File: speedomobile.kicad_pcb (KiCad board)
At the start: 2 copper layers, 100 x 100 mm, 126 parts, among them J1 Conn_01x04, J10 Conn_02x02_Odd_Even, J11 Conn_02x02_Odd_Even, J12 Conn_02x02_Odd_Even, J13 Conn_02x02_Odd_Even, J14 Conn_02x02_Odd_Even, J15 Conn_02x02_Odd_Even, J16 Conn_02x02_Odd_Even, J17 Conn_02x02_Odd_Even, J18 Conn_01x02, J19 Conn_01x02, J2 Conn_01x04, J20 Conn_01x02, J21 Conn_01x02, J22 Conn_01x07, J23 Conn_01x04, J24 Conn_01x03, J25 Conn_01x03, J26 Conn_01x03, J27 Conn_01x02, J28 Conn_01x06, J29 Conn_01x02, J3 Conn_01x04, J30 Conn_01x06, J31 Conn_02x06_Odd_Even, J32 Conn_01x02, J33 Conn_01x03, J34 Conn_01x02, J35 SDCARD_breakout, J36 Conn_02x02_Odd_Even, J37 Conn_01x02, J38 Conn_01x04, J39 Conn_02x02_Odd_Even, J4 Conn_01x04, J5 Conn_01x05, J6 Conn_01x04, J7 Conn_01x07, J8 Conn_01x03, J9 Conn_Coaxial, Q1 DMT6012LSS, Q2 DMT6012LSS, SW1 SW_Push, U1 MCP1501-33xCH, U10 NEO-M9N, U11 PCF8574, U12 PCF8574, U13 TCA9617A, U2 SC0918, U3 74AHCT367, U4 BTS4140N, U5 CD74HC4067M, U6 MCS1802, U7 MCS1802, U8 V48SD, U9 adafruit_LSM9DS1

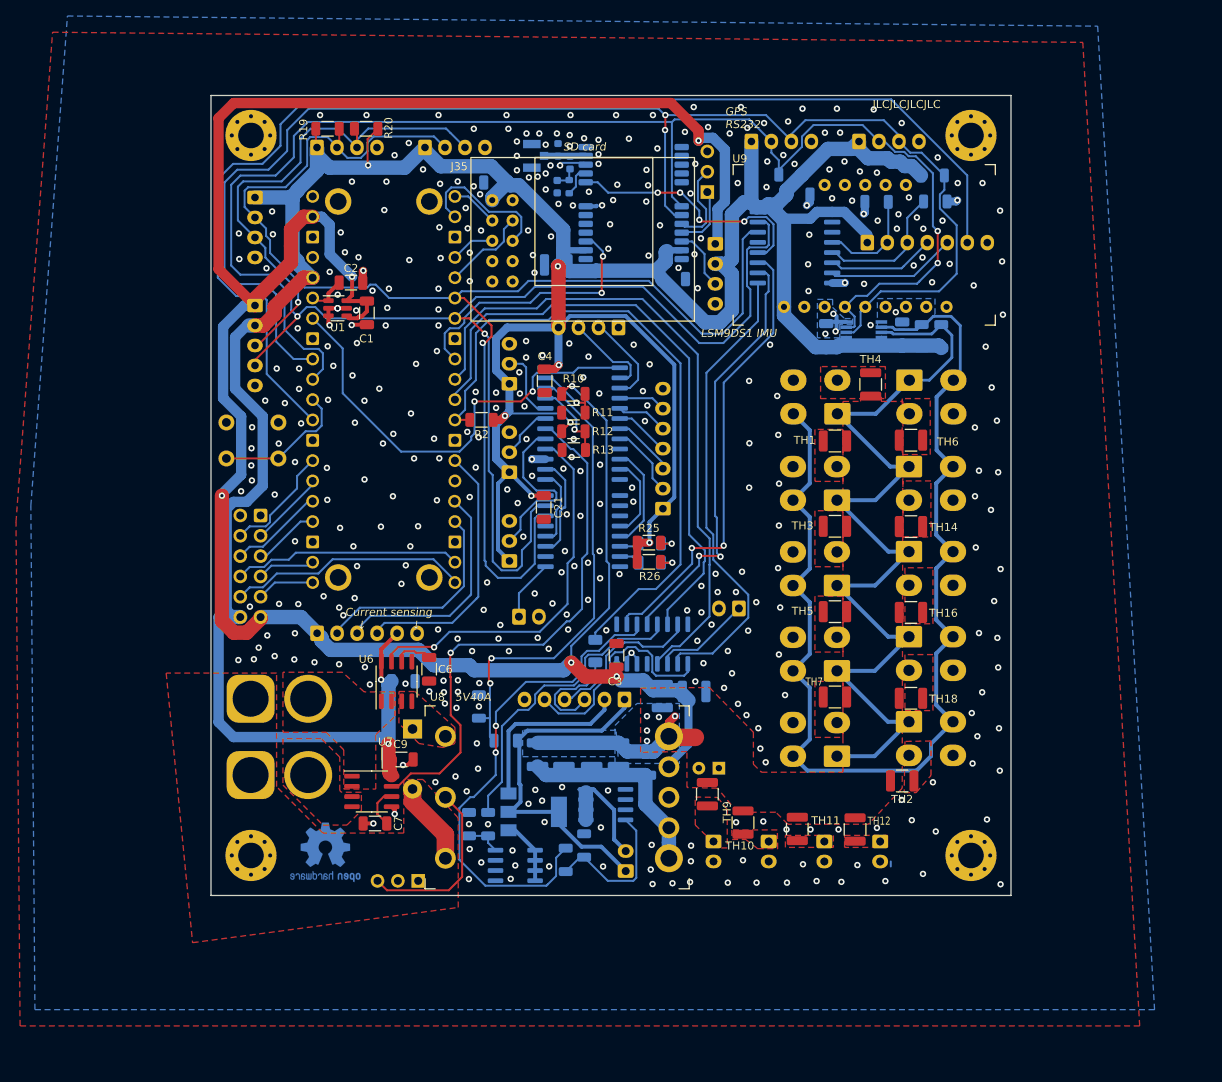
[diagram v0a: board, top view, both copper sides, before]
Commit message: Prepare for merging
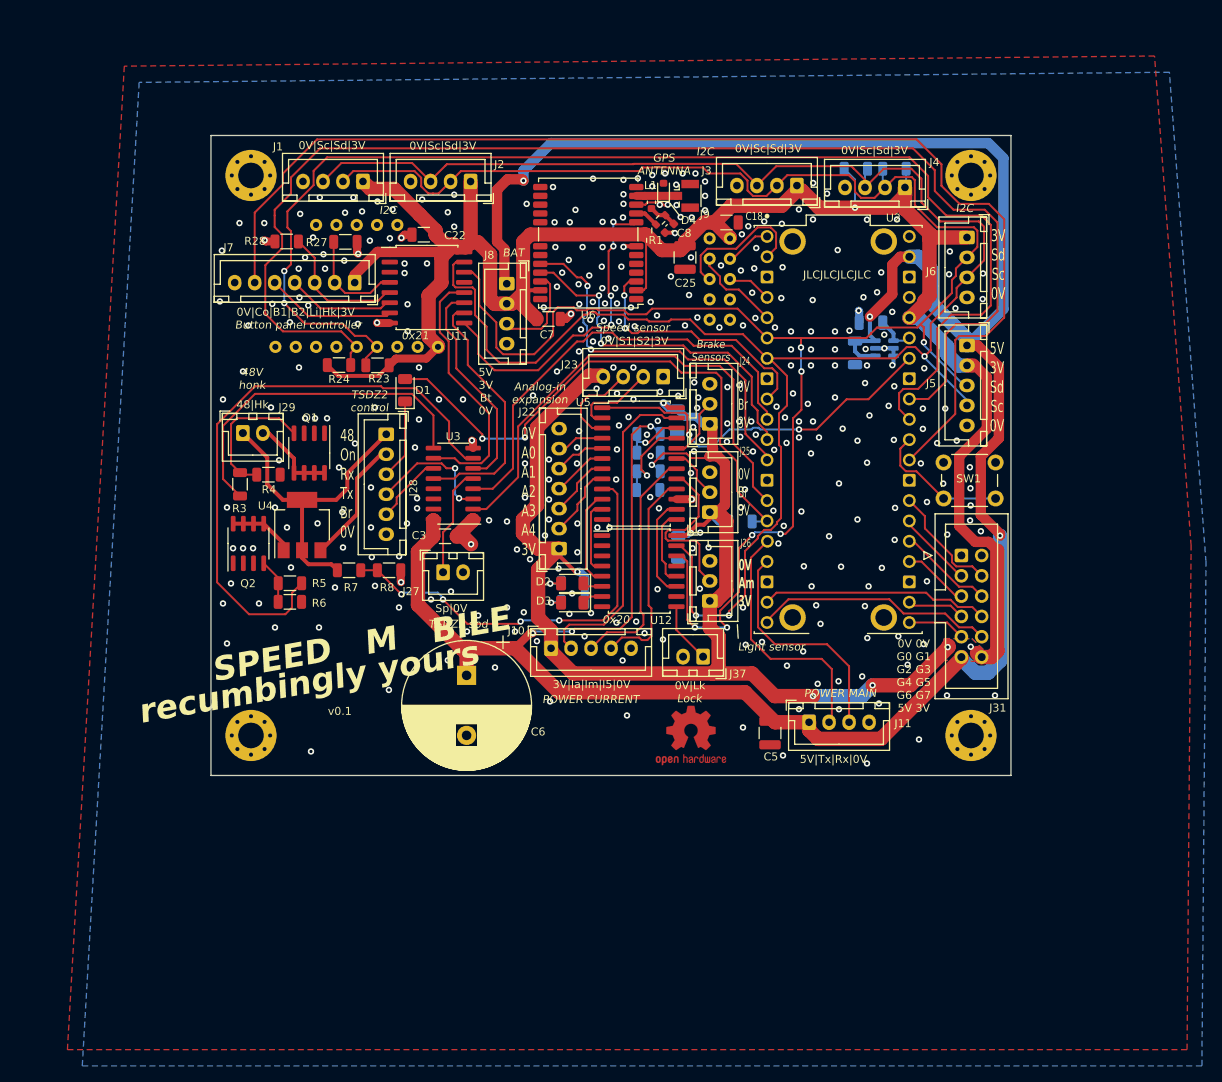
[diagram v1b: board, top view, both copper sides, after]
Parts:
- removed C10, C11, C12, C13, C15, C16: 22u, Capacitor_SMD:C_1210_3225Metric
- removed C14: 100u, Capacitor_THT:CP_Radial_D6.3mm_P2.50mm
- removed C19, C9: 1u, Capacitor_SMD:C_1206_3216Metric
- removed C20: 100n, Capacitor_SMD:C_0603_1608Metric
- removed C23, C24: 100n, Capacitor_SMD:C_1206_3216Metric
- removed J12, J13, J14, J15, J16, J17, J36, J39: Conn_02x02_Odd_Even, Connector_Molex:Molex_Mini-Fit_Jr_5566-04A_2x02_P4.20mm_Vertical
- removed J18, J19, J20, J21: Conn_01x02, Connector_JST:JST_XH_B2B-XH-A_1x02_P2.50mm_Vertical
- removed J30: Conn_01x06, Connector_JST:JST_XH_B6B-XH-A_1x06_P2.50mm_Vertical
- removed J32: Conn_01x02, Connector_AMASS:AMASS_XT60-M_1x02_P7.20mm_Vertical
- removed J33: Conn_01x03, Connector_PinHeader_2.54mm:PinHeader_1x03_P2.54mm_Vertical
- removed J34: Conn_01x02, Connector_AMASS:AMASS_XT60-F_1x02_P7.20mm_Vertical
- removed J38: Conn_01x04, Connector_JST:JST_XH_B4B-XH-A_1x04_P2.50mm_Vertical
- removed R18: 20, Resistor_SMD:R_0603_1608Metric
- removed R29: 330, Resistor_SMD:R_1206_3216Metric
- removed TH1, TH14, TH16, TH18, TH2, TH3, TH4, TH5, TH6, TH7: 7,5A, Resistor_SMD:R_1210_3225Metric
- removed TH10, TH11, TH12, TH13, TH9: 3A, Resistor_SMD:R_1210_3225Metric
- removed U10: NEO-M9N, RF_GPS:ublox_NEO
- removed U13: TCA9617A, Package_SO:VSSOP-8_3.0x3.0mm_P0.65mm
- removed U7: MCS1802, Package_SO:SOIC-8_3.9x4.9mm_P1.27mm
- removed U8: V48SD, additional:V48D
- C1, C2, C21, C4, H1, H2, H3, H4, J35, R10, R11, R12, R13, R19, R2, R20, R25, R26, U1, U9: moved to B.Cu
- C18, C22, C25, D1, D2, D3, D4, J1, J2, J22, J27, J28, J29, J3, J31, J37, J4, J5, J6, J7, J9, L1, Q1, Q2, R23, R24, R27, R28, R3, R4, R5, R6, R7, R8, SW1, SYMB1, U11, U12, U2, U3, U4, U5: moved to F.Cu
- C5: value 220u -> 22u; footprint Capacitor_THT:CP_Radial_D16.0mm_P7.50mm -> Capacitor_SMD:C_1210_3225Metric; moved to F.Cu
- C6: value 1u -> 220u; footprint Capacitor_SMD:C_1206_3216Metric -> Capacitor_THT:CP_Radial_D16.0mm_P7.50mm
- C8: value 1u -> 100n; footprint Capacitor_SMD:C_1206_3216Metric -> Capacitor_SMD:C_0603_1608Metric; moved to F.Cu
- J10: value Conn_02x02_Odd_Even -> Conn_01x05; footprint Connector_Molex:Molex_Mini-Fit_Jr_5566-04A_2x02_P4.20mm_Vertical -> Connector_JST:JST_XH_B5B-XH-A_1x05_P2.50mm_Vertical; moved to F.Cu
- J11: value Conn_02x02_Odd_Even -> JST_XH; footprint Connector_Molex:Molex_Mini-Fit_Jr_5566-04A_2x02_P4.20mm_Vertical -> Connector_JST:JST_XH_B4B-XH-A_1x04_P2.50mm_Vertical; moved to F.Cu
- J23: value Conn_01x04 -> XHB4B; moved to F.Cu
- J24, J25, J26: value Conn_01x03 -> XHB3B; moved to F.Cu
- J8: value Conn_01x03 -> Conn_01x04; footprint Connector_PinHeader_2.54mm:PinHeader_1x03_P2.54mm_Vertical -> Connector_JST:JST_XH_B4B-XH-A_1x04_P2.50mm_Vertical; moved to F.Cu
- R1: value 330 -> 20; footprint Resistor_SMD:R_1206_3216Metric -> Resistor_SMD:R_0603_1608Metric; moved to F.Cu
- U6: value MCS1802 -> NEO-M9N; footprint Package_SO:SOIC-8_3.9x4.9mm_P1.27mm -> RF_GPS:ublox_NEO
- moved H1 91.2 mm to (180.0, 110.0), turned to 180 degrees
- moved H2 91.2 mm to (90.0, 110.0), turned to 180 degrees
- moved H3 90.1 mm to (90.0, 40.0), turned to 180 degrees
- moved H4 90.1 mm to (180.0, 40.0), turned to 180 degrees
- moved J5 89.1 mm to (179.5, 61.2)
- moved J6 89.1 mm to (179.5, 47.8)
- moved J31 87.7 mm to (178.8, 87.5), turned to 0 degrees
- moved SW1 83.3 mm to (176.6, 75.9), turned to 0 degrees
- moved R28 81.2 mm to (94.5, 48.2), turned to 180 degrees
- moved R24 77.9 mm to (101.0, 63.7)
- moved J4 73.7 mm to (171.8, 41.5), turned to 180 degrees
- moved J29 72.7 mm to (89.0, 72.2), turned to 0 degrees
- moved R19 71.0 mm to (170.4, 39.2), turned to 180 degrees
- moved U1 68.5 mm to (169.2, 61.6), turned to 180 degrees
- moved C7 66.7 mm to (127.2, 57.9), turned to 0 degrees
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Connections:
- net /VREF renamed +3.3VA
- net Net-(J29-Pin_2) renamed /HONK_48V
- C5 pad 1: /power/Dcdc -> +5VL
- C5 pad 2: -BATT -> GND
- C6 pad 1: Net-(U6-FILTER) -> +5VL
- C7 pad 1: Net-(U7-FILTER) -> +3V3
- C8 pad 1: +3V3 -> Net-(C8-Pad1)
- D4 pad 1: /I2C devices/RF_GPS -> /GPS/RF_GPS
- J1 pad 2: /FAST_SDA -> /SDA
- J1 pad 3: /FAST_SCL -> /SCL
- J10 pad 1: /I2C devices/led ribbon/FAST_SCL_5V -> +3V3
- J10 pad 2: /I2C devices/led ribbon/LED1 -> /Analog input/Iaux
- J10 pad 3: /I2C devices/led ribbon/FAST_SDA_5V -> /Analog input/Imotor
- J10 pad 4: GND -> /Analog input/I5V
- J11 pad 1: /I2C devices/led ribbon/FAST_SCL_5V -> +5VL
- J11 pad 2: /I2C devices/led ribbon/LED2 -> /UARTTX
- J11 pad 3: /I2C devices/led ribbon/FAST_SDA_5V -> /UARTRX
- J2 pad 2: /FAST_SDA -> /SDA
- J2 pad 3: /FAST_SCL -> /SCL
- J8 pad 1: Net-(J8-Pin_1) -> +5VL
- J8 pad 2: Net-(J8-Pin_2) -> +3V3
- J8 pad 3: GND -> Net-(J8-Pin_3)
- J9 pad 1: /I2C devices/RF_GPS -> /GPS/RF_GPS
- L1 pad 1: Net-(C20-Pad1) -> Net-(C8-Pad1)
- L1 pad 2: /I2C devices/RF_GPS -> /GPS/RF_GPS
- R1 pad 1: +3V3 -> Net-(U6-VCC_RF)
- R1 pad 2: /I2C devices/led ribbon/FAST_SCL_5V -> Net-(C8-Pad1)
- U11 pad 10: /TSDZ2_ON -> /TSDZ2_BRAKE
- U11 pad 11: /HONK -> /TSDZ2_ON
- U11 pad 12: /I2C devices/RESET_M9N -> /HONK
- U11 pad 9: /TSDZ2_BRAKE -> /RESET_M9N
- U2 pad 11: /TSDZ2_TX -> /GPS_TX
- U2 pad 12: /TSDZ2_RX -> /GPS_RX
- U2 pad 14: /AUX -> /TSDZ2_TX
- U2 pad 15: unconnected-(U2-I2C1SCL/SPI1TX/GP11-Pad15) -> /TSDZ2_RX
- U3 pad 10: /TSDZ2_BRAKE -> /HONK
- U3 pad 11: /VSPEED_5V -> /TSDZ2_BRAKE_5V
- U3 pad 12: /VSPEED -> /TSDZ2_BRAKE
- U3 pad 2: /HONK -> /TSDZ2_TX
- U3 pad 3: /HONK_5V -> /TSDZ2_TX_5V
- U3 pad 4: /TSDZ2_ON -> /VSPEED
- U3 pad 5: /TSDZ2_ON_5V -> /VSPEED_5V
- U3 pad 6: /TSDZ2_TX -> /TSDZ2_ON
- U3 pad 7: /TSDZ2_TX_5V -> /TSDZ2_ON_5V
- U3 pad 9: /TSDZ2_BRAKE_5V -> /HONK_5V
- U5 pad 16: /I5V -> /Analog input/I5V
- U5 pad 18: /Imotor -> /Analog input/Imotor
- U5 pad 2: /Analog input/ADC_SPEED1 -> /Analog input/ADC_SPEED2
- U5 pad 22: /Analog input/VBATADC -> /Analog input/U5V
- U5 pad 23: /Analog input/U5V -> /Analog input/Iaux
- U5 pad 3: /Analog input/ADC_SPEED2 -> /Analog input/ADC_SPEED1
- U5 pad 9: unconnected-(U5-I0-Pad9) -> /Analog input/VBATADC
- U6 pad 1: +BATT -> unconnected-(U6-~{SAFEBOOT}-Pad1)
- U6 pad 2: +BATT -> +3V3
- U6 pad 3: /power/Dcdc -> /PPS
- U6 pad 4: /power/Dcdc -> unconnected-(U6-EXTINT-Pad4)
- U6 pad 5: GND -> unconnected-(U6-USB_DM-Pad5)
- U6 pad 6: Net-(U6-FILTER) -> unconnected-(U6-USB_DP-Pad6)
- U6 pad 7: /I5V -> GND
- U6 pad 8: +3V3 -> /RESET_M9N
- U9 pad 6: GND -> unconnected-(U9-CS_AG-Pad6)
- U9 pad 7: GND -> unconnected-(U9-CS_M-Pad7)
- U9 pad 8: GND -> unconnected-(U9-MISO_AG-Pad8)
- U9 pad 9: GND -> unconnected-(U9-MISO_M-Pad9)
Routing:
- net /I2C devices/led ribbon/FAST_SDA_5V: track 141.9 -> 0.00 mm
- net /I2C devices/led ribbon/FAST_SCL_5V: track 119.6 -> 0.00 mm
- net /Imotor: track 67.6 -> 0.00 mm, vias 1 -> 0
- net /SDA: track 184.4 -> 251.9 mm, vias 2 -> 7
- net /SCL: track 192.9 -> 254.8 mm, vias 2 -> 3
- net /GPS_RX: track 0.00 -> 47.8 mm, vias 0 -> 2
- net /I5V: track 47.4 -> 0.00 mm, vias 1 -> 0
- net /GPS_TX: track 0.00 -> 44.7 mm, vias 0 -> 2
- net /RESET_M9N: track 0.00 -> 40.9 mm, vias 0 -> 4
- net /Analog input/Iaux: track 0.00 -> 40.7 mm
- net /TSDZ2_ON_5V: track 38.6 -> 73.9 mm
- net /AUX: track 33.3 -> 0.00 mm
- net /I2C devices/RESET_M9N: track 31.8 -> 0.00 mm, vias 4 -> 0
- net /Analog input/Imotor: track 0.00 -> 29.8 mm
- net GND: track 58.7 -> 29.6 mm, vias 392 -> 353
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- added copper zone on B.Cu, net +3V3
- added copper zone on F.Cu, net +3V3
- removed copper zone on B.Cu, net +5V
- removed copper zone on F.Cu, net +5V
- removed copper zone on F.Cu, net +BATT
- removed copper zone on F.Cu, net -BATT
- removed copper zone on F.Cu, net /I2C devices/led ribbon/LED1
- removed copper zone on F.Cu, net /I2C devices/led ribbon/LED10
- removed copper zone on F.Cu, net /I2C devices/led ribbon/LED2
- removed copper zone on F.Cu, net /I2C devices/led ribbon/LED3
- removed copper zone on F.Cu, net /I2C devices/led ribbon/LED4
- removed copper zone on F.Cu, net /I2C devices/led ribbon/LED5
- removed copper zone on F.Cu, net /I2C devices/led ribbon/LED6
- removed copper zone on F.Cu, net /I2C devices/led ribbon/LED7
- removed copper zone on F.Cu, net /I2C devices/led ribbon/LED8
- removed copper zone on F.Cu, net /I2C devices/led ribbon/LED9
- removed copper zone on F.Cu, net /power/Dcdc
- removed copper zone on F.Cu, net /power/Motor
- removed copper zone on F.Cu, net /power/PWR1
- removed copper zone on F.Cu, net /power/PWR2
- removed copper zone on F.Cu, net /power/PWR3
- removed copper zone on F.Cu, net /power/PWR4
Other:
- board size 100 x 100 mm -> 100 x 80 mm
- board text added: "0V 0V G0 G1 G2 G3 G4 G5 G6 G7 5V 3V"
- board text added: "0V A0 A1 A2 A3 A4 3V"
- board text added: "0V Am 3V"
- board text added: "0V Br 3V"
- board text added: "0V|Co|B1|B2|Li|Hk|3V"
- board text added: "0V|Lk"
- board text added: "0V|S1|S2|3V"
- board text added: "0V|Sc|Sd|3V"
- board text added: "0x20"
- board text added: "0x21"
- board text added: "3V Sd Sc 0V"
- board text added: "3V|Ia|Im|I5|0V"
- board text added: "48 On Rx Tx Br 0V"
- board text added: "48|Hk"
- board text added: "5V 3V Bt 0V"
- board text added: "5V 3V Sd Sc 0V"
- board text added: "5V|Tx|Rx|0V"
- board text added: "Brake Sensors"
- board text added: "I2C"
- board text added: "LSM9DS1 IMU (I2C 0x6A 0x1C)"
- board text added: "POWER CURRENT"
- board text added: "POWER MAIN"
- board text added: "Sp|0V"
- board text added: "TSDZ2 spd"
- board text removed: "5V On/Off"
- board text removed: "5V-7.5A I2C"
- board text removed: "5V40A"
- board text removed: "Battery"
- board text removed: "Brake sensor x2"
- board text removed: "Current sensing ↓ ↓"
- board text removed: "Fast-I2C expansion"
- board text removed: "GPS RS232"
- board text removed: "I2C Expansion"
- board text removed: "I2C expansion"
- board text removed: "LCD+RFID"
- board text removed: "LSM9DS1 IMU"
- board text removed: "Motor"
- board text removed: "TSDZ2 speed return"
- board text removed: "uart+aux"
